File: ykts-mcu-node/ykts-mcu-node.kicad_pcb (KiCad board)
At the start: 2 copper layers, 16.8 x 13.5 mm, 22 parts, among them J1 PWEN, J2 RX, J3 TX, J4 ~RST, J5 GND, J6 VCC, J7 VCC, J8 GND, SW1 ADG802BRT, U1 ATmega328PB-MU, Y1 8 MHz

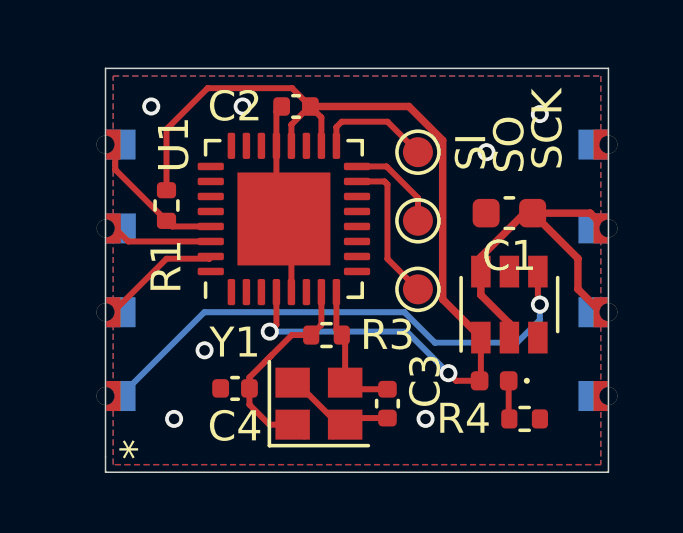
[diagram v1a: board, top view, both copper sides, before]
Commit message: Hierarchal sheet rework
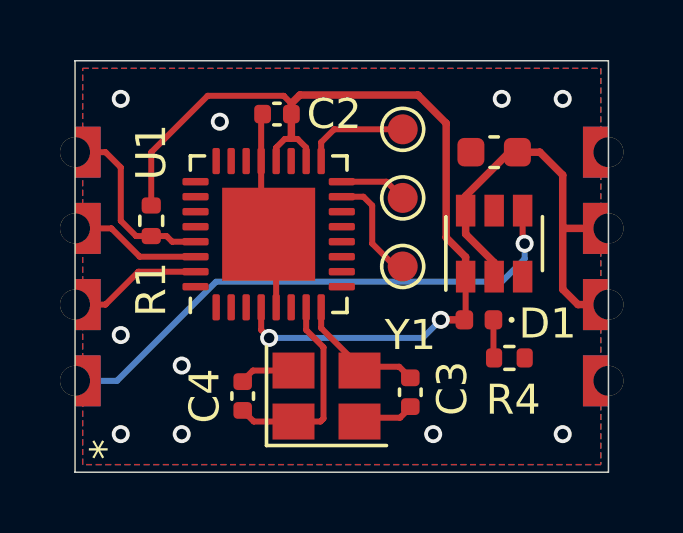
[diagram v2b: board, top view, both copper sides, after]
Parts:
- removed R3: 1M, Resistor_SMD:R_0402_1005Metric
- J1, J4, J5, J6, J7, J8: footprint ykts-mcu-node:CastellatedHole_0.6mm -> ykts-mcu-node:CastellatedHole_1.0mm
- J2: value RX -> TX; footprint ykts-mcu-node:CastellatedHole_0.6mm -> ykts-mcu-node:CastellatedHole_1.0mm
- J3: value TX -> RX; footprint ykts-mcu-node:CastellatedHole_0.6mm -> ykts-mcu-node:CastellatedHole_1.0mm
- Y1: footprint Crystal:Crystal_SMD_2520-4Pin_2.5x2.0mm -> Crystal:Crystal_SMD_3225-4Pin_3.2x2.5mm
- moved D1 2.09 mm to (115.6, 85.3)
- moved C1 2.09 mm to (116.1, 79.8)
- moved R4 2.09 mm to (116.6, 86.6)
- moved SW1 2.09 mm to (116.1, 82.8)
- moved J1 1.14 mm to (102.1, 87.4)
- moved J2 1.05 mm to (102.1, 84.8)
- moved J4 1.05 mm to (102.1, 79.8)
- moved J3 1.02 mm to (102.1, 82.3)
- moved TP1 0.92 mm to (113.0, 81.3)
- moved TP2 0.92 mm to (113.0, 83.6)
- moved TP3 0.92 mm to (113.0, 79.0)
- moved C3 0.85 mm to (113.3, 87.8)
- moved R1 0.72 mm to (104.6, 82.0)
- moved U1 0.72 mm to (108.6, 82.5)
- moved C2 0.68 mm to (108.8, 78.5)
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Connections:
- SW1 pad 5: Net-(SW1-Pad5) -> (no net)
- U1 pad 1: Net-(U1-Pad1) -> (no net)
- U1 pad 10: Net-(U1-Pad10) -> (no net)
- U1 pad 11: Net-(U1-Pad11) -> (no net)
- U1 pad 12: Net-(U1-Pad12) -> (no net)
- U1 pad 13: Net-(U1-Pad13) -> (no net)
- U1 pad 14: Net-(U1-Pad14) -> (no net)
- U1 pad 19: Net-(U1-Pad19) -> (no net)
- U1 pad 2: Net-(U1-Pad2) -> (no net)
- U1 pad 22: Net-(U1-Pad22) -> (no net)
- U1 pad 23: Net-(U1-Pad23) -> (no net)
- U1 pad 24: Net-(U1-Pad24) -> (no net)
- U1 pad 25: Net-(U1-Pad25) -> (no net)
- U1 pad 26: Net-(U1-Pad26) -> (no net)
- U1 pad 27: Net-(U1-Pad27) -> (no net)
- U1 pad 28: Net-(U1-Pad28) -> (no net)
- U1 pad 3: Net-(U1-Pad3) -> (no net)
- U1 pad 32: Net-(U1-Pad32) -> (no net)
- U1 pad 6: Net-(U1-Pad6) -> (no net)
- U1 pad 9: Net-(U1-Pad9) -> (no net)
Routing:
- net Net-(C2-Pad1): track 33.2 -> 31.0 mm
- net +5V: track 12.4 -> 13.9 mm
- net /ISP_MOSI: track 4.97 -> 3.74 mm
- net /ISP_RESET: track 4.80 -> 5.87 mm
- net Net-(C4-Pad1): track 7.87 -> 6.83 mm
- net /ISP_MISO: track 3.23 -> 2.25 mm
- net /UART0_RX: track 3.36 -> 3.98 mm
- net GND: track 11.1 -> 10.7 mm, vias 7 -> 10
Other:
- board size 16.8 x 13.5 mm -> 17.8 x 13.7 mm
- board text removed: "SCK"
- board text removed: "SI"
- board text removed: "SO"
